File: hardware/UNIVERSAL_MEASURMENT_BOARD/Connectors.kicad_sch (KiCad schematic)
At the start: 44 parts, among them J1 FTSH-107-01-L-D-K, J2 2606-1110_010-000, J3 2606-1110_010-000, J4 Conn_01x01_Socket, J5 Conn_01x01_Socket, J6 Conn_01x01_Socket, J7 Conn_01x01_Socket, J8 2606-1110_010-000, J9 2606-1110_010-000, U16 ESDS304DBVR, U17 ESDS304DBVR

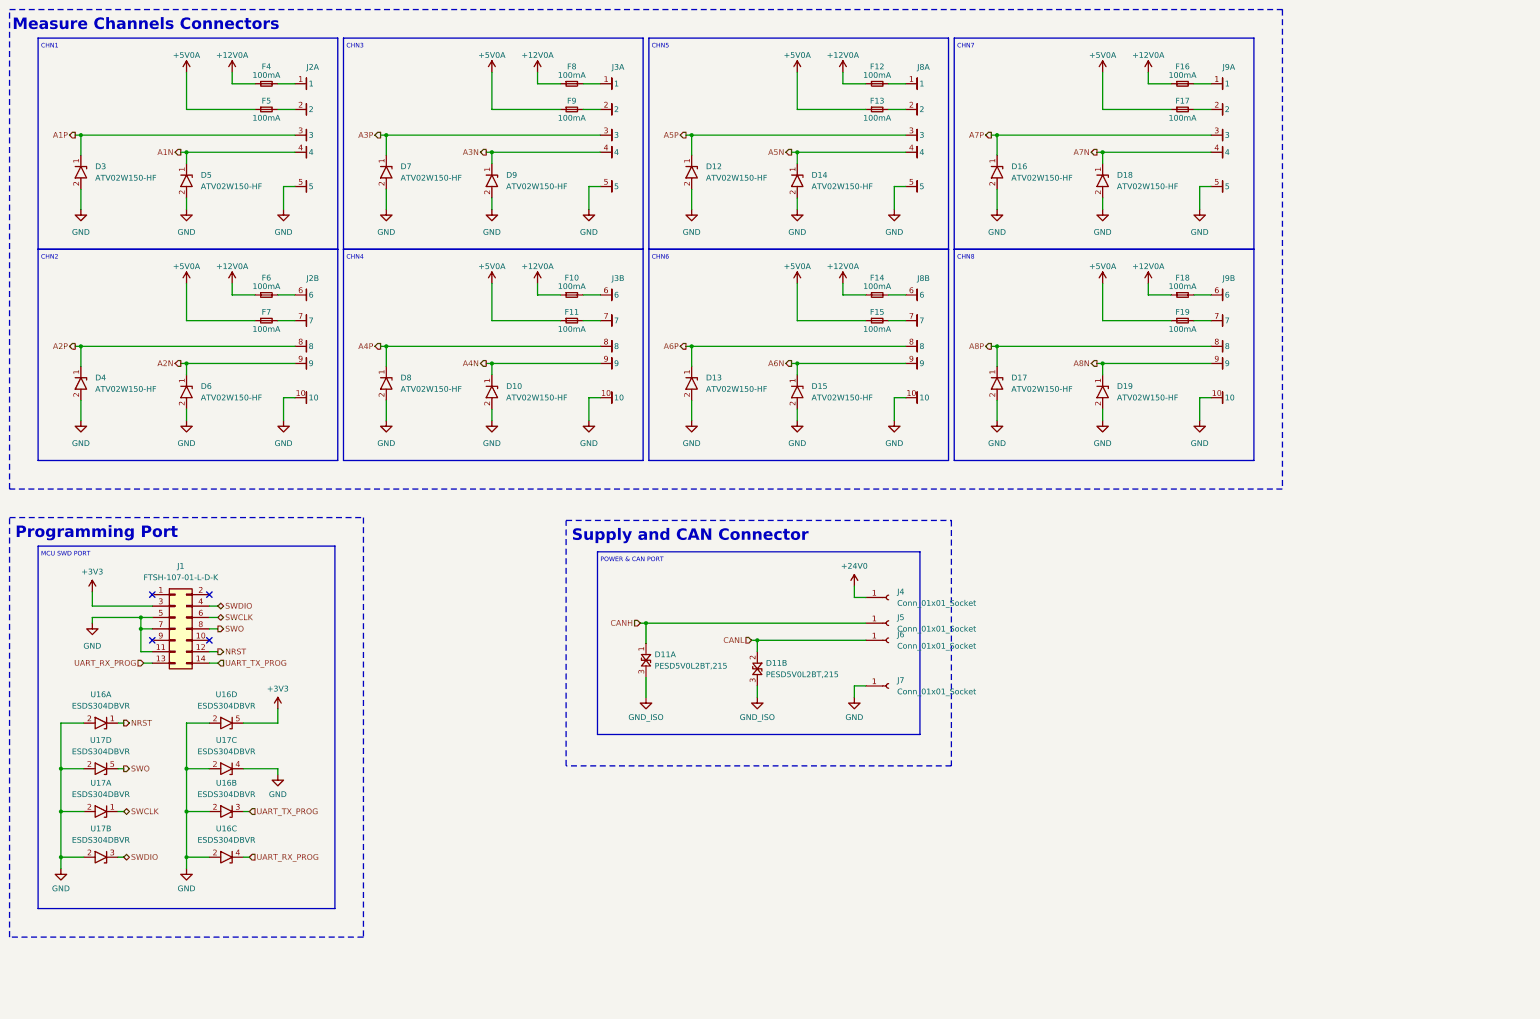
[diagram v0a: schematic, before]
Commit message: clean up project visuals
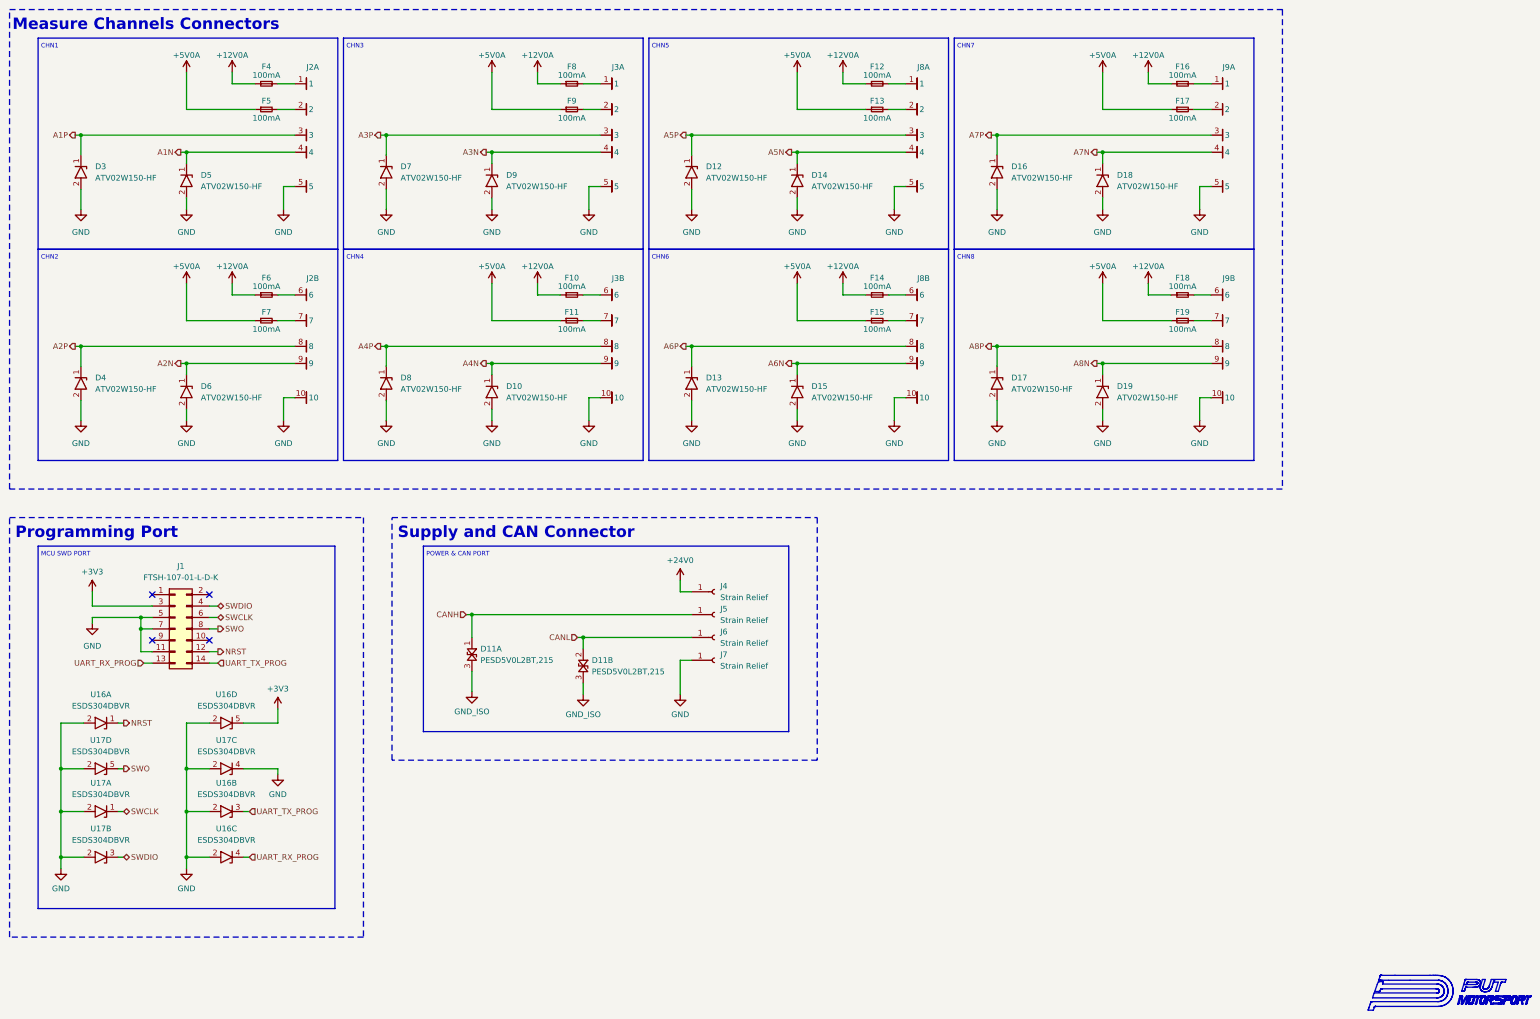
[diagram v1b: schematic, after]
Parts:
- J4, J5, J6, J7: value Conn_01x01_Socket -> Strain Relief
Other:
- moved on the sheet: D11A, D11B, J4, J5, J6, J7
